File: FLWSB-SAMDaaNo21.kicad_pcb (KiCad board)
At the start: 2 copper layers, 51.4 x 18.5 mm, 36 parts, among them J1 USB4085-GF-A_REVA4, J2 DEBUG, J3 Conn_01x15_Male, J4 Conn_01x15_Male, SW1 SW_RESET, U1 LD1117S33TR_SOT223, U2 ATSAMD21G18A-A, Y1 Crystal_Small

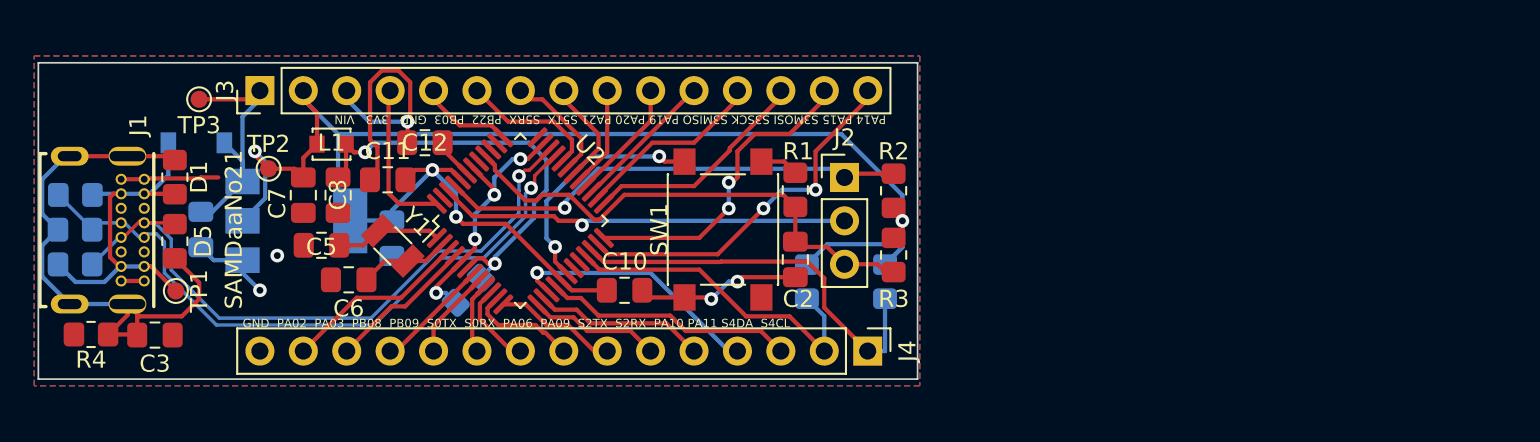
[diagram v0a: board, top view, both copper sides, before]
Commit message: Laatste verbeteringen
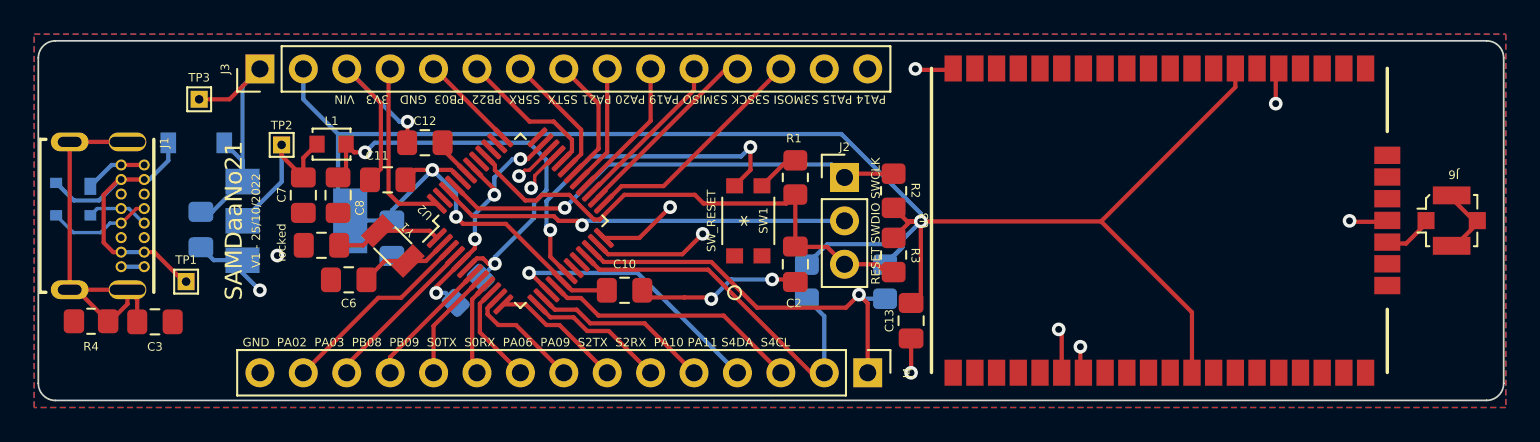
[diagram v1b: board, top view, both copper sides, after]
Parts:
- removed D2, D3, D4, D5: D_Zener, Resistor_SMD:R_0805_2012Metric_Pad1.20x1.40mm_HandSolder
- added C13: 1µF, Capacitor_SMD:C_0805_2012Metric_Pad1.18x1.45mm_HandSolder, F.Cu at (134.6, 84.6)
- added J6: Conn_Coaxial, Connector_Coaxial:U.FL_Molex_MCRF_73412-0110_Vertical, F.Cu at (166.2, 78.7)
- added U3: RN2483, RN2483:RN2483, F.Cu at (149.1, 78.7)
- D1: value D_Zener -> PRTR5V0U2X; footprint Resistor_SMD:R_0805_2012Metric_Pad1.20x1.40mm_HandSolder -> Package_TO_SOT_SMD:SOT-143; moved to B.Cu
- SW1: footprint Button_Switch_SMD:SW_Push_1P1T_NO_6x6mm_H9.5mm -> KMR7_CNK:KMR7_CNK
- TP1, TP2, TP3: footprint TestPoint:TestPoint_Pad_D1.0mm -> TestPoint:TestPoint_THTPad_1.0x1.0mm_Drill0.5mm
- moved D1 6.08 mm to (85.6, 77.5), turned to 180 degrees
- moved TP2 1.59 mm to (97.8, 74.3)
- moved SW1 1.57 mm to (125.1, 78.7), turned to 90 degrees
- moved J3 1.27 mm to (96.5, 69.8)
- moved J4 1.27 mm to (132.1, 87.6)
- moved J1 0.84 mm to (85.7, 78.4)
- moved TP1 0.81 mm to (92.2, 82.3)
- moved C3 0.77 mm to (90.4, 84.6)
- moved R4 0.77 mm to (86.6, 84.6)
- moved R1 0.73 mm to (127.8, 76.2)
- moved C2 0.28 mm to (127.8, 81.3)
- renumbered C5 to locked
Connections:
- net PA09 renamed PA07
- net PA10 renamed RN2483_RESET
- D1 pad 1: VBUS -> GND
- D1 pad 2: Net-(C3-Pad2) -> USB-
- SW1 pad 1: Net-(R1-Pad1) -> unconnected-(SW1-Pad1)
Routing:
- net RN2483_RESET: track 14.9 -> 56.3 mm, vias 1 -> 2
- net VDDIN: track 95.0 -> 134.9 mm, vias 4 -> 3
- net SERCOM2_PAD1_TX: track 7.75 -> 35.9 mm, vias 0 -> 1
- net SERCOM2_PAD2_RX: track 10.1 -> 35.5 mm, vias 0 -> 1
- net GND: track 67.8 -> 80.1 mm, vias 11 -> 14
- net Net-(C3-Pad2): track 34.4 -> 22.9 mm
- net USB-: track 38.8 -> 30.2 mm
- net USB+: track 38.4 -> 32.3 mm
- net VBUS: track 22.0 -> 19.0 mm
- net 868MHz: track 0.00 -> 2.75 mm
- net VIN: track 14.7 -> 17.2 mm
- net SERCOM4_PAD0_SDA: track 19.7 -> 21.5 mm
- net PA20: track 5.36 -> 7.14 mm
- net PA19: track 6.62 -> 8.40 mm
- net PA21: track 5.79 -> 7.57 mm
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- added copper zone on In1.Cu, net GND
- added copper zone on In2.Cu, net VDDIN
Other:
- board size 51.4 x 18.5 mm -> 85.7 x 21 mm
- copper layers 2 -> 4
- board text added: "RESET SWDIO SWCLK"
- board text added: "V1 - 25/10/2022"
